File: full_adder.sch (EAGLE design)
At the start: 73 parts, among them IC1 SN74LS74AN, IC2 NE555, IC3 CD4052BE, IC4 CD4052BE, IC5 CD4052BE, IC6 74HC4051N,652, U1 ATTINY45-20P

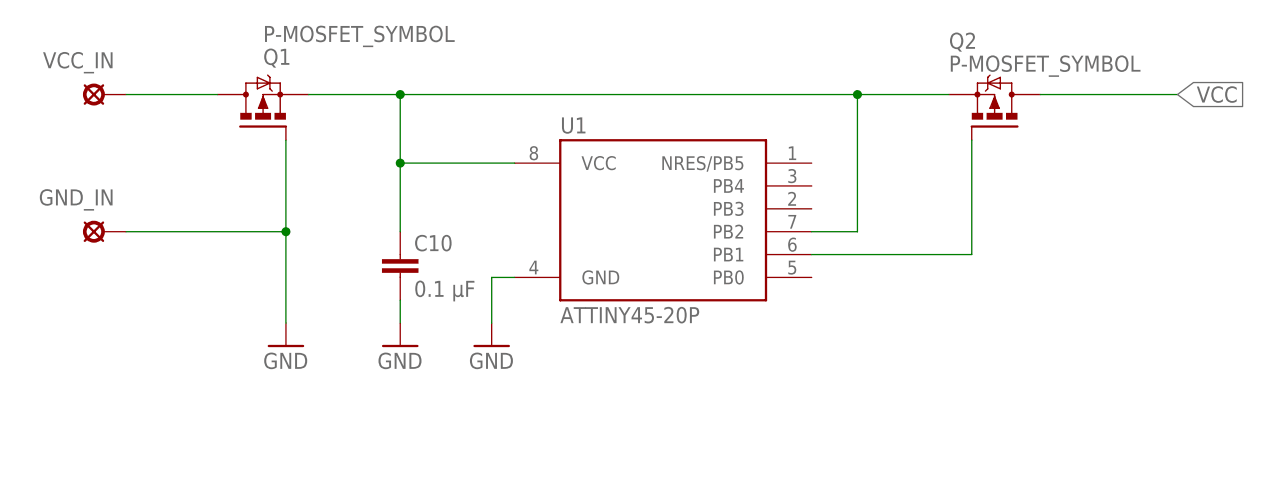
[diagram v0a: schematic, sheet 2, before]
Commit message: minor fixes
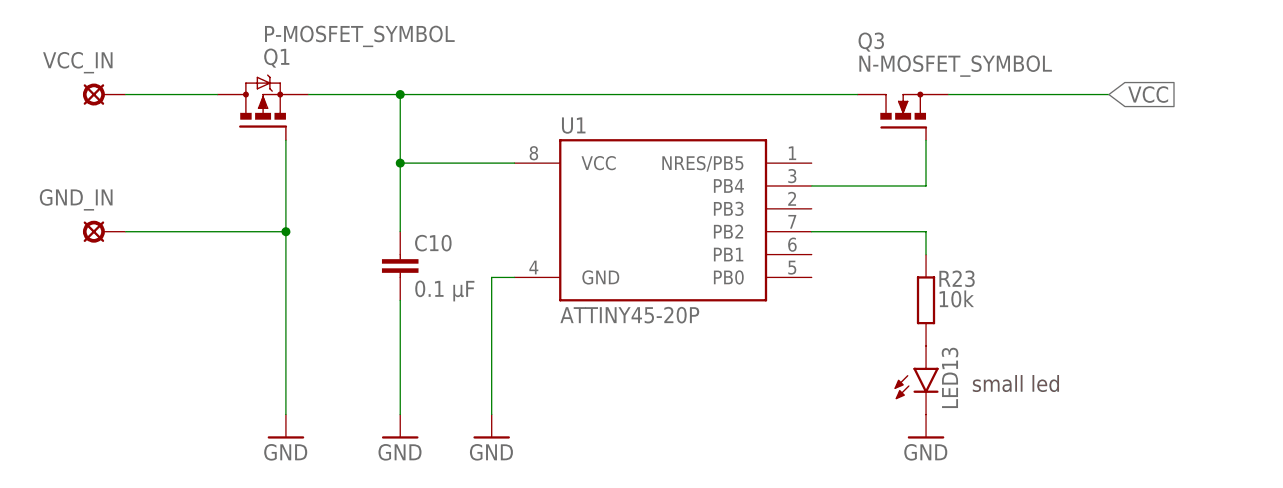
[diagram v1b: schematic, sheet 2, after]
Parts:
- added LED13: (no value), led:LED5MM
- added R23: 10k, rcl:R-EU_R1206
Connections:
- new net N$33: LED13.A, R23.1
- new net N$34: R23.2, U1.PB2
- net GND: now also LED13.C
- net N$31: no longer U1.PB2
- net N$32: now also U1.PB4; no longer U1.PB1
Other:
- note added: "small led"
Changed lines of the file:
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@@
 <part name="C10" library="rcl" library_urn="urn:adsk.eagle:library:334" deviceset="C-EU" device="025-024X044" package3d_urn="urn:adsk.eagle:package:23630/1" value="0.1 µF"/>
 <part name="GND49" library="supply1" library_urn="urn:adsk.eagle:library:371" deviceset="GND" device=""/>
-<part name="Q2" library="transistor-power" library_urn="urn:adsk.eagle:library:400" deviceset="P-MOSFET_SYMBOL" device=""/>
+<part name="Q3" library="transistor-power" library_urn="urn:adsk.eagle:library:400" deviceset="N-MOSFET_SYMBOL" device=""/>
+<part name="LED13" library="led" library_urn="urn:adsk.eagle:library:259" deviceset="LED" device="5MM" package3d_urn="urn:adsk.eagle:package:15799/2"/>
+<part name="R23" library="rcl" library_urn="urn:adsk.eagle:library:334" deviceset="R-EU_" device="R1206" package3d_urn="urn:adsk.eagle:package:23540/2" value="10k"/>
+<part name="GND50" library="supply1" library_urn="urn:adsk.eagle:library:371" deviceset="GND" device=""/>
 </parts>
 <sheets>
@@
 <plain>
 <text x="-177.8" y="190.5" size="3.81" layer="100">10 Reverse Polarity + Overdischarge Protection</text>
+<text x="-73.66" y="144.78" size="1.778" layer="97">small led</text>
 </plain>
 <instances>
@@
 <attribute name="NAME" x="-168.91" y="167.259" size="1.778" layer="95" rot="R180"/>
 </instance>
-<instance part="GND47" gate="1" x="-149.86" y="149.86" smashed="yes">
-<attribute name="VALUE" x="-152.4" y="147.32" size="1.778" layer="96"/>
+<instance part="GND47" gate="1" x="-149.86" y="139.7" smashed="yes">
+<attribute name="VALUE" x="-152.4" y="137.16" size="1.778" layer="96"/>
 </instance>
 <instance part="Q1" gate="G$1" x="-152.4" y="175.26" smashed="yes" rot="MR90">
@@
 <attribute name="VALUE" x="-119.38" y="152.4" size="1.778" layer="96"/>
 </instance>
-<instance part="GND48" gate="1" x="-127" y="149.86" smashed="yes">
-<attribute name="VALUE" x="-129.54" y="147.32" size="1.778" layer="96"/>
+<instance part="GND48" gate="1" x="-127" y="139.7" smashed="yes">
+<attribute name="VALUE" x="-129.54" y="137.16" size="1.778" layer="96"/>
 </instance>
 <instance part="C10" gate="G$1" x="-137.16" y="160.02" smashed="yes">
@@
 <attribute name="VALUE" x="-135.636" y="155.321" size="1.778" layer="96"/>
 </instance>
-<instance part="GND49" gate="1" x="-137.16" y="149.86" smashed="yes">
-<attribute name="VALUE" x="-139.7" y="147.32" size="1.778" layer="96"/>
-</instance>
-<instance part="Q2" gate="G$1" x="-71.12" y="175.26" smashed="yes" rot="R90">
-<attribute name="NAME" x="-76.2" y="182.88" size="1.778" layer="95"/>
-<attribute name="VALUE" x="-76.2" y="180.34" size="1.778" layer="96"/>
+<instance part="GND49" gate="1" x="-137.16" y="139.7" smashed="yes">
+<attribute name="VALUE" x="-139.7" y="137.16" size="1.778" layer="96"/>
+</instance>
+<instance part="Q3" gate="G$1" x="-81.28" y="175.26" smashed="yes" rot="R90">
+<attribute name="NAME" x="-86.36" y="182.88" size="1.778" layer="95"/>
+<attribute name="VALUE" x="-86.36" y="180.34" size="1.778" layer="96"/>
+</instance>
+<instance part="LED13" gate="G$1" x="-78.74" y="147.32" smashed="yes">
+<attribute name="NAME" x="-75.184" y="142.748" size="1.778" layer="95" rot="R90"/>
+<attribute name="VALUE" x="-73.025" y="142.748" size="1.778" layer="96" rot="R90"/>
+</instance>
+<instance part="R23" gate="G$1" x="-78.74" y="154.94" smashed="yes" rot="R90">
+<attribute name="NAME" x="-77.47" y="156.4386" size="1.778" layer="95"/>
+<attribute name="VALUE" x="-77.47" y="154.178" size="1.778" layer="96"/>
+</instance>
+<instance part="GND50" gate="1" x="-78.74" y="139.7" smashed="yes">
+<attribute name="VALUE" x="-81.28" y="137.16" size="1.778" layer="96"/>
 </instance>
 </instances>
@@
 <wire x1="-149.86" y1="162.56" x2="-167.64" y2="162.56" width="0.1524" layer="91"/>
 <pinref part="GND47" gate="1" pin="GND"/>
-<wire x1="-149.86" y1="152.4" x2="-149.86" y2="162.56" width="0.1524" layer="91"/>
+<wire x1="-149.86" y1="142.24" x2="-149.86" y2="162.56" width="0.1524" layer="91"/>
 <junction x="-149.86" y="162.56"/>
 </segment>
@@
 <pinref part="U1" gate="G$1" pin="GND"/>
 <wire x1="-124.46" y1="157.48" x2="-127" y2="157.48" width="0.1524" layer="91"/>
-<wire x1="-127" y1="157.48" x2="-127" y2="152.4" width="0.1524" layer="91"/>
+<wire x1="-127" y1="157.48" x2="-127" y2="142.24" width="0.1524" layer="91"/>
 <pinref part="GND48" gate="1" pin="GND"/>
 </segment>
@@
 <pinref part="GND49" gate="1" pin="GND"/>
 <pinref part="C10" gate="G$1" pin="2"/>
-<wire x1="-137.16" y1="152.4" x2="-137.16" y2="154.94" width="0.1524" layer="91"/>
+<wire x1="-137.16" y1="142.24" x2="-137.16" y2="154.94" width="0.1524" layer="91"/>
+</segment>
+<segment>
+<pinref part="GND50" gate="1" pin="GND"/>
+<pinref part="LED13" gate="G$1" pin="C"/>
 </segment>
 </net>
@@
 <wire x1="-137.16" y1="170.18" x2="-124.46" y2="170.18" width="0.1524" layer="91"/>
 <wire x1="-137.16" y1="177.8" x2="-86.36" y2="177.8" width="0.1524" layer="91"/>
-<wire x1="-86.36" y1="177.8" x2="-86.36" y2="162.56" width="0.1524" layer="91"/>
 <junction x="-137.16" y="177.8"/>
-<pinref part="U1" gate="G$1" pin="PB2"/>
-<wire x1="-86.36" y1="162.56" x2="-91.44" y2="162.56" width="0.1524" layer="91"/>
 <pinref part="C10" gate="G$1" pin="1"/>
 <wire x1="-137.16" y1="162.56" x2="-137.16" y2="170.18" width="0.1524" layer="91"/>
 <junction x="-137.16" y="170.18"/>
-<wire x1="-86.36" y1="177.8" x2="-76.2" y2="177.8" width="0.1524" layer="91"/>
-<junction x="-86.36" y="177.8"/>
+</segment>
+</net>
+<net name="VCC" class="0">
+<segment>
+<wire x1="-76.2" y1="177.8" x2="-58.42" y2="177.8" width="0.1524" layer="91"/>
+<label x="-58.42" y="177.8" size="1.778" layer="95" xref="yes"/>
 </segment>
 </net>
 <net name="N$32" class="0">
 <segment>
-<pinref part="U1" gate="G$1" pin="PB1"/>
-<wire x1="-91.44" y1="160.02" x2="-73.66" y2="160.02" width="0.1524" layer="91"/>
-<wire x1="-73.66" y1="172.72" x2="-73.66" y2="160.02" width="0.1524" layer="91"/>
-</segment>
-</net>
-<net name="VCC" class="0">
-<segment>
-<wire x1="-66.04" y1="177.8" x2="-50.8" y2="177.8" width="0.1524" layer="91"/>
-<label x="-50.8" y="177.8" size="1.778" layer="95" xref="yes"/>
-</segment>
-</net>
+<pinref part="U1" gate="G$1" pin="PB4"/>
+<wire x1="-91.44" y1="167.64" x2="-78.74" y2="167.64" width="0.1524" layer="91"/>
+<wire x1="-78.74" y1="167.64" x2="-78.74" y2="172.72" width="0.1524" layer="91"/>
+</segment>
+</net>
+<net name="N$33" class="0">
+<segment>
+<pinref part="R23" gate="G$1" pin="1"/>
+<pinref part="LED13" gate="G$1" pin="A"/>
+</segment>
+</net>
+<net name="N$34" class="0">
+<segment>
+<pinref part="U1" gate="G$1" pin="PB2"/>
+<wire x1="-91.44" y1="162.56" x2="-78.74" y2="162.56" width="0.1524" layer="91"/>
+<pinref part="R23" gate="G$1" pin="2"/>
+<wire x1="-78.74" y1="162.56" x2="-78.74" y2="160.02" width="0.1524" layer="91"/>
+</segment>
+</net>
